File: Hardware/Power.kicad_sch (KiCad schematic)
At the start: 21 parts, among them J1 Conn_01x02_Pin, J17 Conn_01x04_Pin, J18 Conn_01x02_Pin, J19 Conn_01x02_Pin, J2 MP1584 Breakout, J20 Conn_01x04_Pin, J3 DRV8833 Breakout, SW1 SW_SPDT, SW2 SW_SPDT

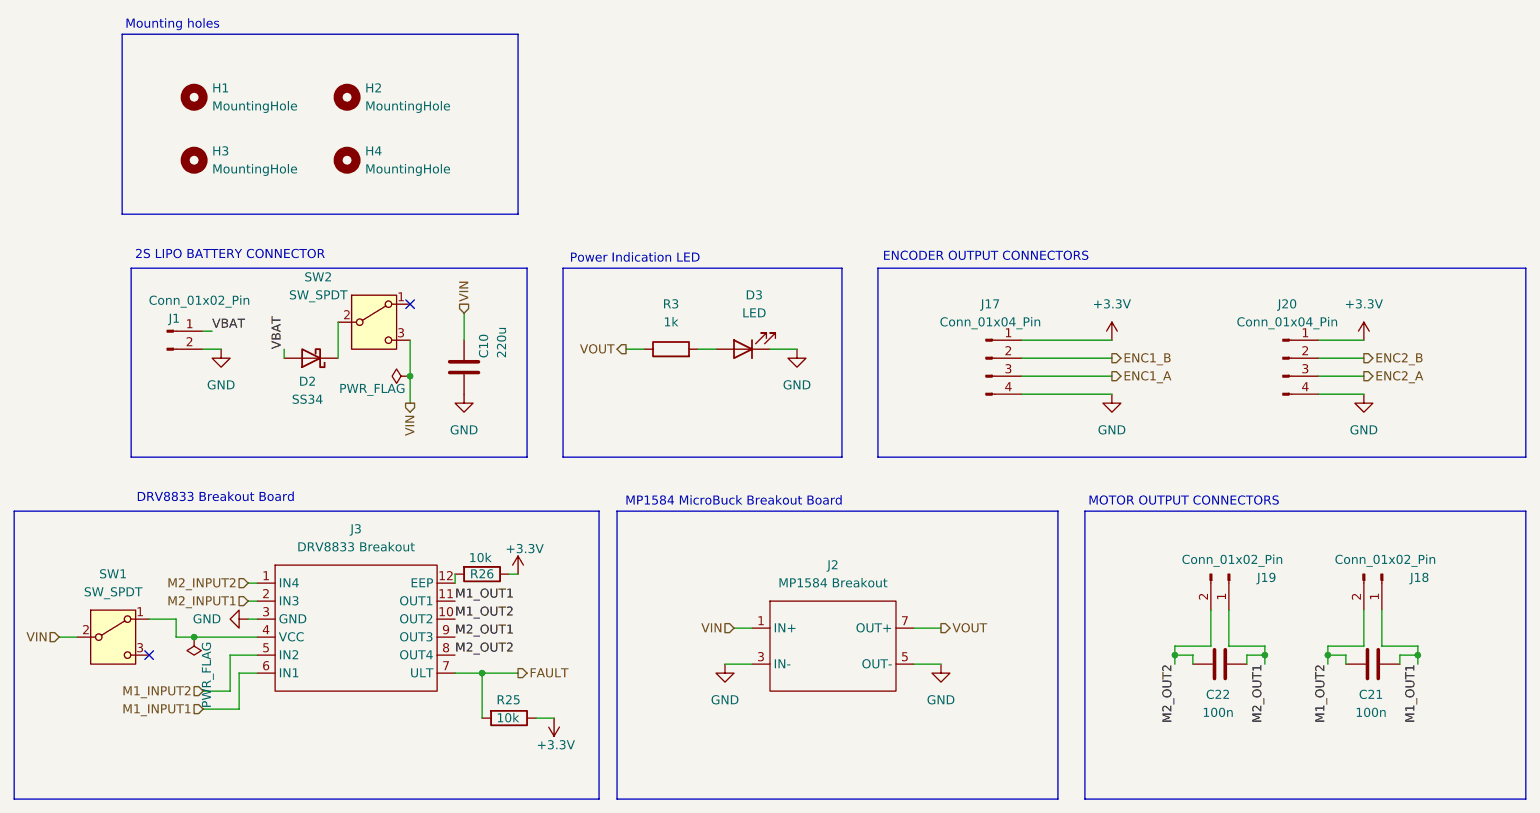
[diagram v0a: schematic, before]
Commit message: Final updated pcb and schematic before dfm check
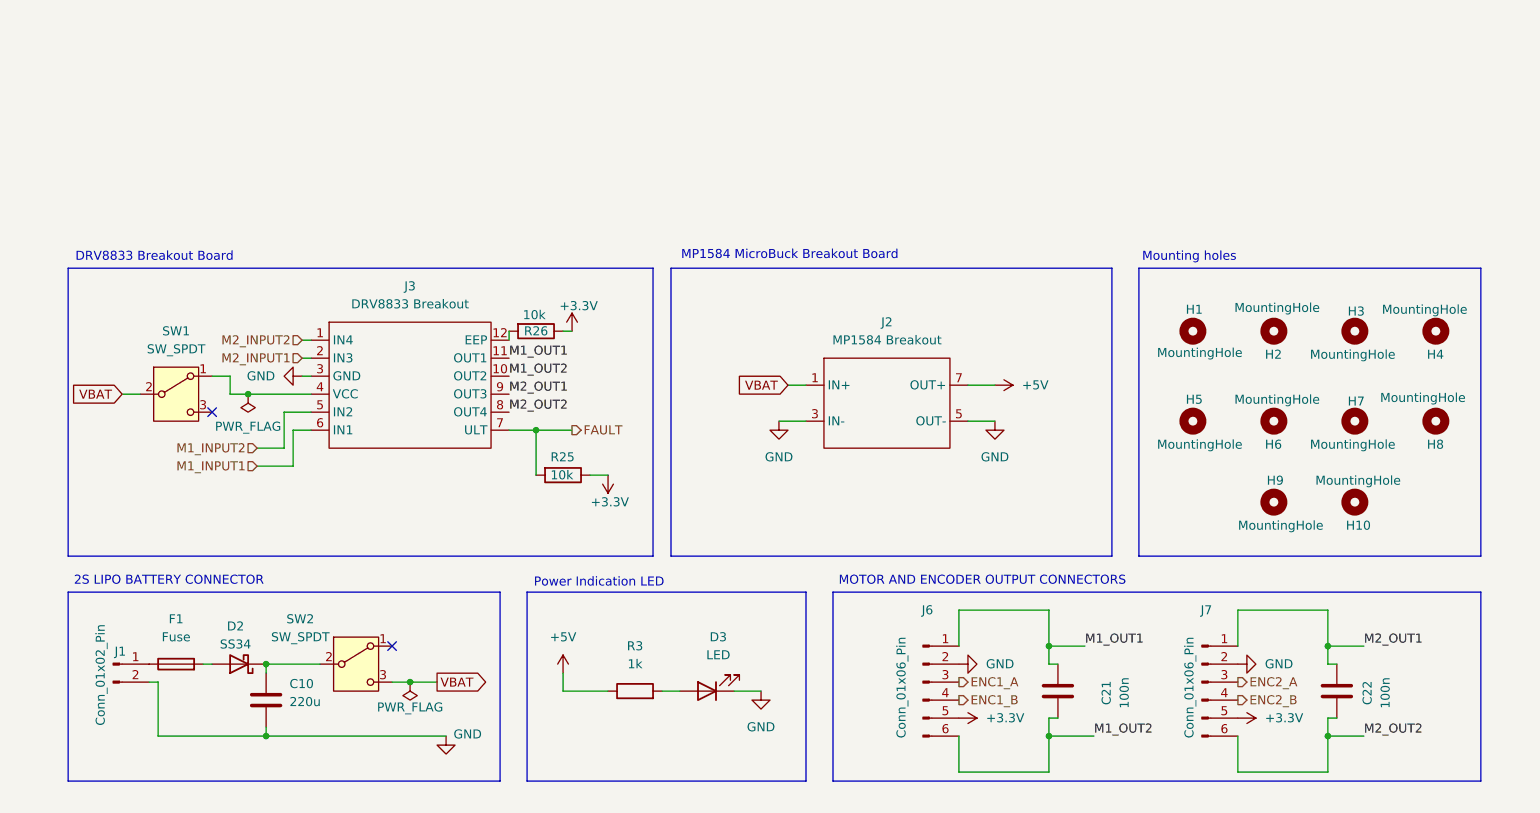
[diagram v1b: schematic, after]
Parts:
- removed J17, J20: Conn_01x04_Pin, Connector_JST:JST_PH_B4B-PH-K_1x04_P2.00mm_Vertical, symbol Connector:Conn_01x04_Pin
- removed J18, J19: Conn_01x02_Pin, Connector_JST:JST_PH_B2B-PH-K_1x02_P2.00mm_Vertical, symbol Connector:Conn_01x02_Pin
- added F1: Fuse, Fuse:Fuse_1206_3216Metric_Pad1.42x1.75mm_HandSolder, symbol Device:Fuse
- added H10, H5, H6, H7, H8, H9: MountingHole, MountingHole:MountingHole_2mm, symbol Mechanical:MountingHole
- added J6, J7: Conn_01x06_Pin, Connector_PinHeader_2.54mm:PinHeader_1x06_P2.54mm_Vertical, symbol Connector:Conn_01x06_Pin
- C10, C21, C22: footprint Capacitor_SMD:C_0603_1608Metric -> Capacitor_SMD:C_0603_1608Metric_Pad1.08x0.95mm_HandSolder
- D2: footprint Diode_SMD:D_SMA -> Diode_SMD:D_SMA_Handsoldering
- D3: footprint LED_SMD:LED_0603_1608Metric -> LED_THT:LED_D3.0mm
- J1: footprint Connector_JST:JST_XH_B2B-XH-A_1x02_P2.50mm_Vertical -> Connector_AMASS:AMASS_XT60-M_1x02_P7.20mm_Vertical
- R25, R26, R3: footprint Resistor_SMD:R_0603_1608Metric -> Resistor_SMD:R_0603_1608Metric_Pad0.98x0.95mm_HandSolder
- SW1, SW2: footprint Button_Switch_SMD:SW_SPDT_CK_JS102011SAQN -> Button_Switch_THT:SW_Slide_SPDT_Angled_CK_OS102011MA1Q
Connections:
- net +3.3V: now also J6.5 (Pin_5), J7.5 (Pin_5)
- net ENC1_A: now also J6.3 (Pin_3)
- net ENC1_B: now also J6.4 (Pin_4)
- net ENC2_A: now also J7.3 (Pin_3)
- net ENC2_B: now also J7.4 (Pin_4)
- net GND: now also J6.2 (Pin_2), J7.2 (Pin_2)
- net IN+: no longer C10.1
- net M1_OUT1: now also J6.1 (Pin_1)
- net M1_OUT2: now also J6.6 (Pin_6)
- net M2_OUT1: now also J7.1 (Pin_1)
- net M2_OUT2: now also J7.6 (Pin_6)
- net at D2.1 (K), SW2.2 (B): now also C10.1
- net VBAT: no longer names the net of D2.2 (A)
- net VBAT: now also F1.2; no longer J1.1 (Pin_1)
- net VOUT renamed +5V
- new net: F1.1, J1.1 (Pin_1)
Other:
- note added: "MOTOR AND ENCODER OUTPUT CONNECTORS"
- note removed: "ENCODER OUTPUT CONNECTORS"
- note removed: "MOTOR OUTPUT CONNECTORS"
- moved on the sheet: C10, C21, C22, D2, D3, H1, H2, H3, H4, J1, J2, J3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
